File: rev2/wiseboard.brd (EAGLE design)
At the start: 42 x 42 mm, 58 parts, among them IC1 LT1945, IC2 LM358, IC3 L79L15, IC4 L78L15, IC5 W25Q, IC8 IC6, IC9 BQ24210DQCT, J1 BAT_CON, J2 SOL_CON, J3 PROG_HEADER, J4 BUT_CON, Q1 IRLM, SW1 SPST_TACT-KMR2, SW2 SPST_TACT-KMR2, U3 ESP-WROOM-03

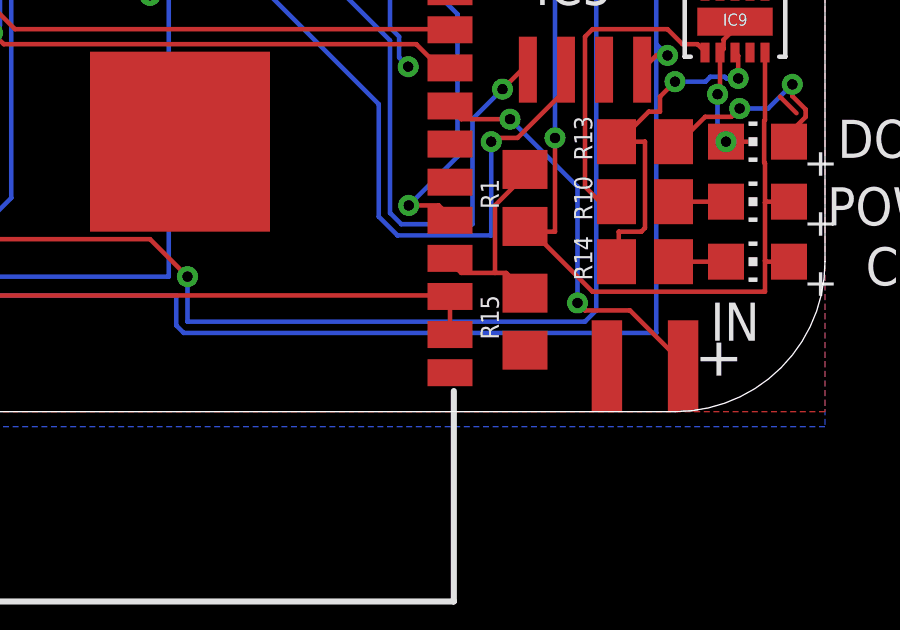
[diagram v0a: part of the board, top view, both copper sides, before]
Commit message: Add test points make to do messages
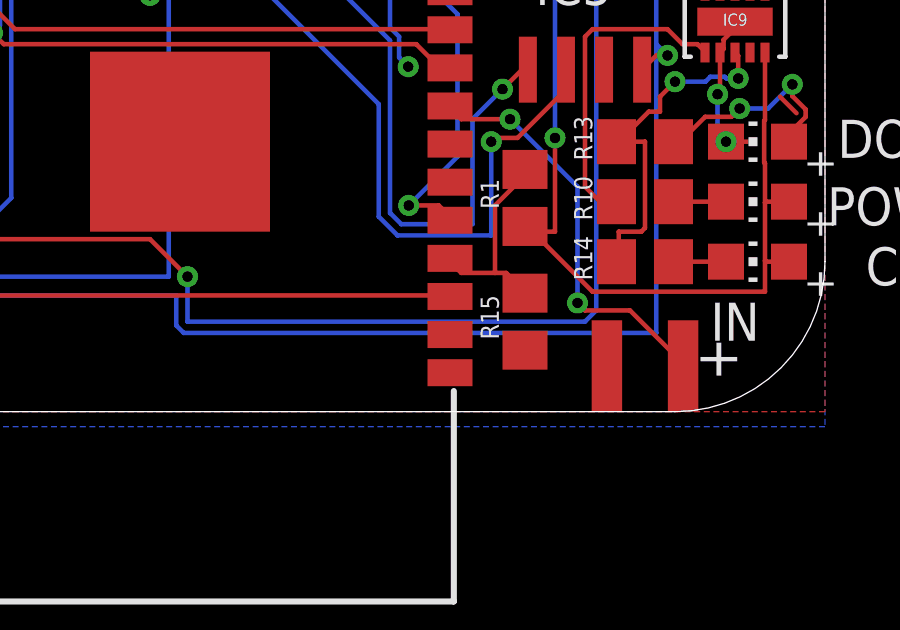
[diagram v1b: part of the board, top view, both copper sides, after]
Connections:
- removed net N$7: U3.25
- net +3V3: no longer U3.3
- net GPIO0: now also U3.25
- net RESET: now also U3.3
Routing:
- net +3V3: track 137.9 -> 136.6 mm
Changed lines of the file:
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@@
 <via x="35.75" y="29.5" extent="1-16" drill="0.35"/>
 <via x="27" y="38.25" extent="1-16" drill="0.35"/>
+<contactref element="U3" pad="25"/>
+<wire x1="11.5" y1="17.81" x2="22" y2="39.2" width="0" layer="19" extent="1-1"/>
 </signal>
 <signal name="RESET">
@@
 <via x="35.75" y="25" extent="1-16" drill="0.35"/>
 <via x="20.125" y="38.875" extent="1-16" drill="0.35"/>
+<contactref element="U3" pad="3"/>
+<wire x1="29.5" y1="3.84" x2="34.5" y2="24.05" width="0" layer="19" extent="1-1"/>
 </signal>
 <signal name="+3V3">
@@
 <contactref element="U$4" pad="P$36"/>
 <contactref element="U$4" pad="P$29"/>
-<contactref element="U3" pad="3"/>
 <contactref element="U3" pad="2"/>
-<wire x1="29.5" y1="3.84" x2="29.5" y2="2.57" width="0.1524" layer="1"/>
 <wire x1="2" y1="4" x2="3.75" y2="4" width="0.1524" layer="1"/>
 <wire x1="1.8" y1="4.2" x2="2" y2="4" width="0.1524" layer="1"/>
@@
 <wire x1="9.639178125" y1="3.875" x2="7.375" y2="3.875" width="0.1524" layer="16"/>
 <wire x1="9.639178125" y1="3.875" x2="12.875" y2="3.875" width="0.1524" layer="16"/>
-<wire x1="29.5" y1="3.875" x2="29.5" y2="3.84" width="0.1524" layer="1"/>
 <wire x1="23.5" y1="33.875" x2="23.25" y2="33.625" width="0.1524" layer="1"/>
 <wire x1="24" y1="33.875" x2="23.5" y2="33.875" width="0.1524" layer="1"/>
@@
 <wire x1="34.0436" y1="38.4564" x2="35.0436" y2="38.4564" width="0.1524" layer="1"/>
 <wire x1="35.0436" y1="38.4564" x2="36.875" y2="36.625" width="0.1524" layer="1"/>
+<wire x1="29.5" y1="3.875" x2="29.5" y2="2.57" width="0" layer="19" extent="1-1"/>
 </signal>
 <signal name="RXD">
@@
 <via x="40" y="17.375" extent="1-16" drill="0.35"/>
 </signal>
-<signal name="N$7">
-<contactref element="U3" pad="25"/>
-</signal>
 <signal name="V+">
